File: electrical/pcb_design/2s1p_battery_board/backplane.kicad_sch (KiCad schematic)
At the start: 37 parts, among them J1 TE_Connectivity_7-5530843-7, J10 TE_Connectivity_7-5530843-7, J11 TE_Connectivity_7-5530843-7, J12 TE_Connectivity_7-5530843-7, J13 TE_Connectivity_7-5530843-7, J14 TE_Connectivity_7-5530843-7, J15 TE_Connectivity_7-5530843-7, J16 TE_Connectivity_7-5530843-7, J2 TE_Connectivity_7-5530843-7, J3 TE_Connectivity_7-5530843-7, J4 TE_Connectivity_7-5530843-7, J5 TE_Connectivity_7-5530843-7, J6 TE_Connectivity_7-5530843-7, J7 TE_Connectivity_7-5530843-7, J8 TE_Connectivity_7-5530843-7, J9 TE_Connectivity_7-5530843-7, U3 TCAN330

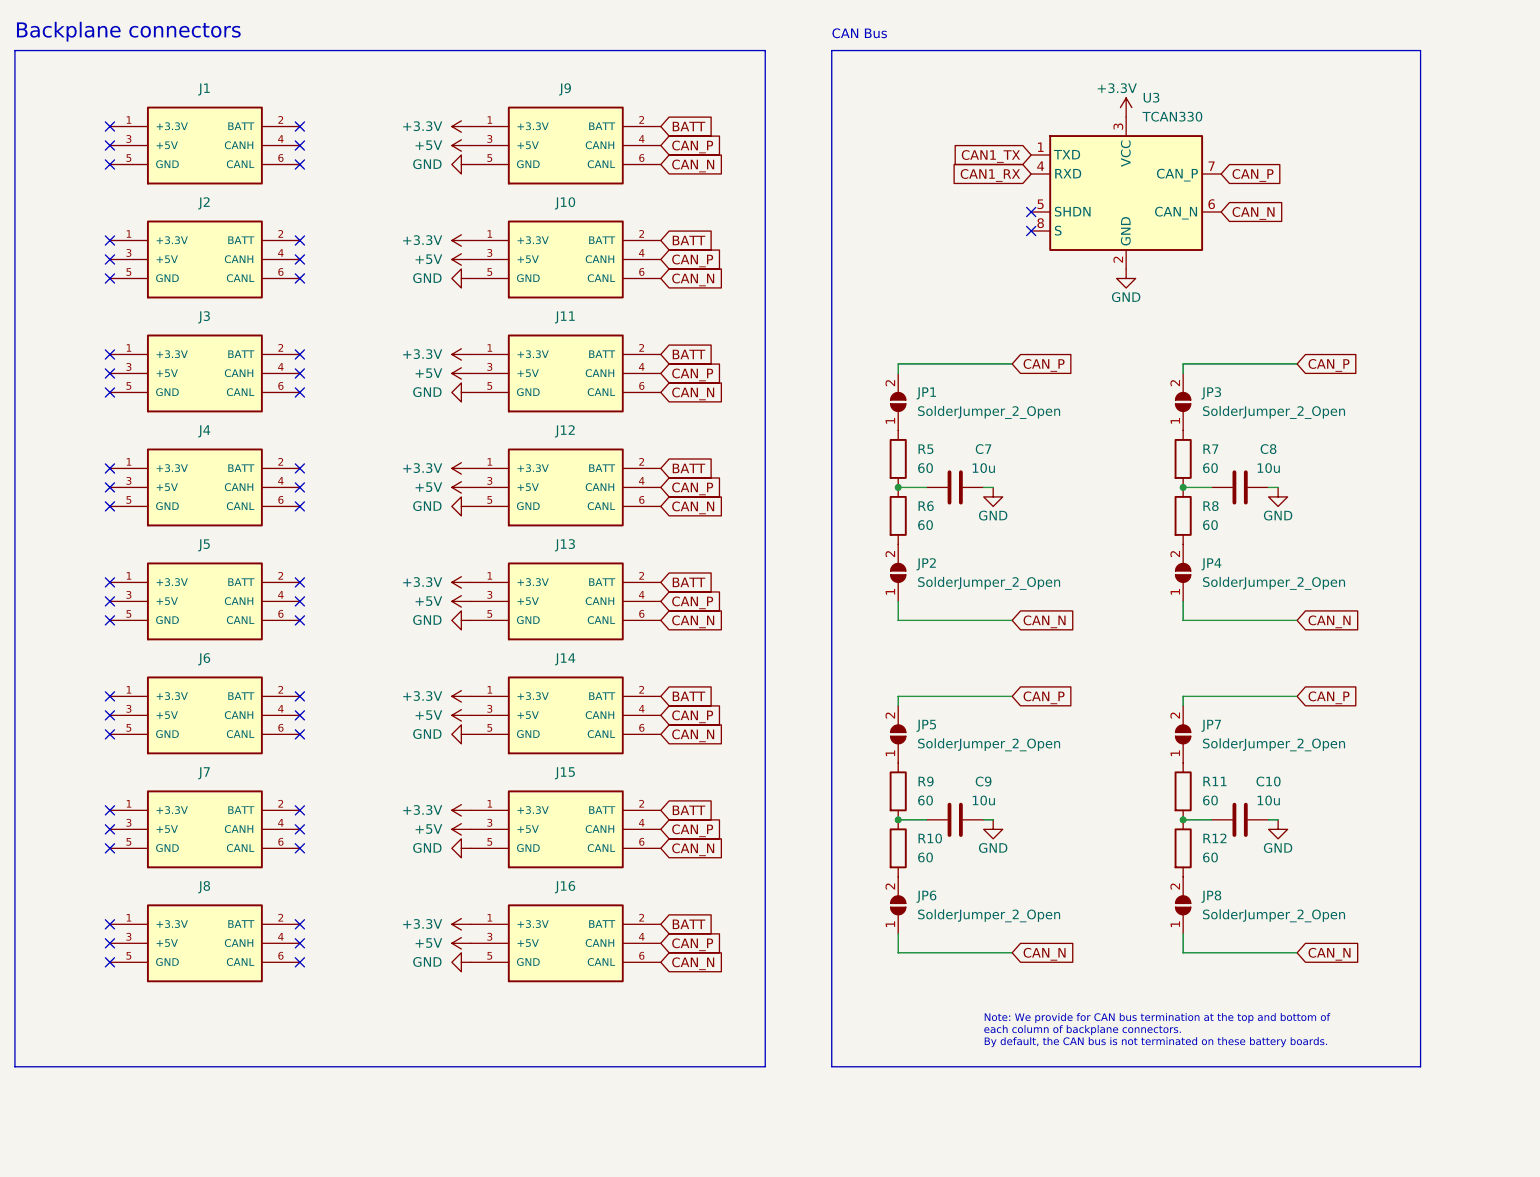
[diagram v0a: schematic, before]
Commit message: Checkpointing work on battery boards
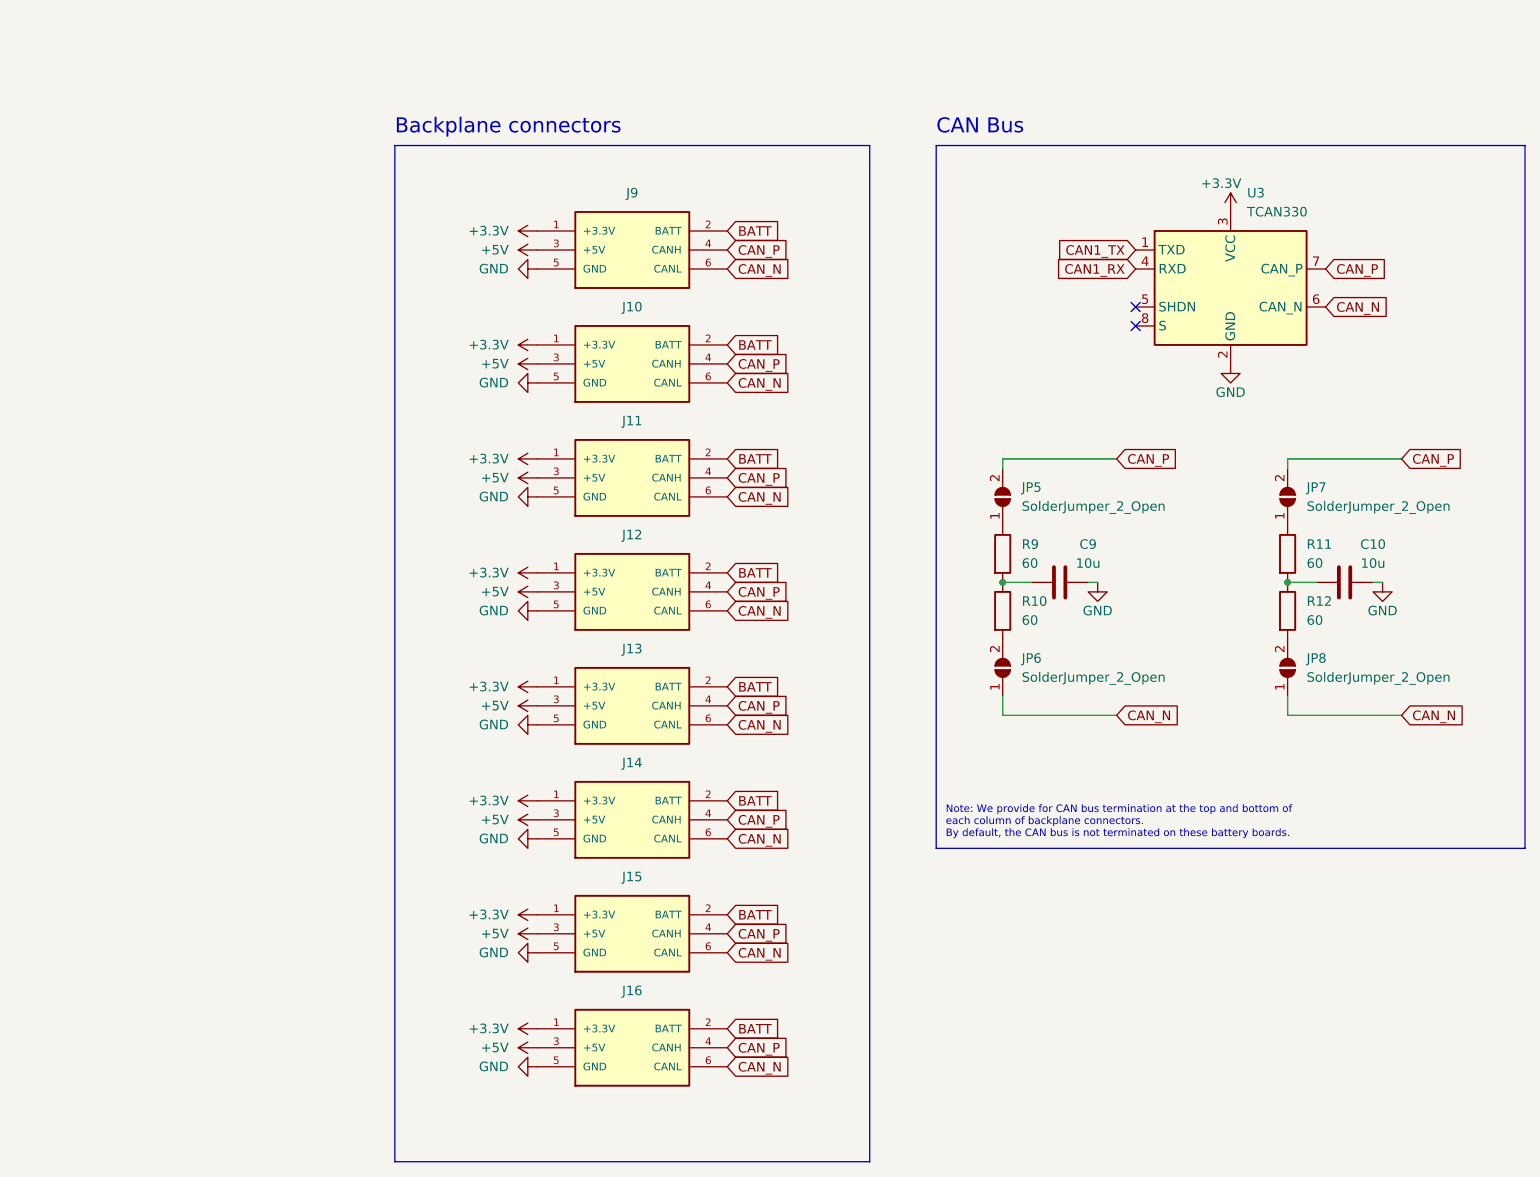
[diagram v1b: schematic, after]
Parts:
- removed C7, C8: 10u, Capacitor_SMD:C_0603_1608Metric, symbol Device:C
- removed J1, J2, J3, J4, J5, J6, J7, J8: TE_Connectivity_7-5530843-7, footprints:TE_Connectivity_7-5530843-7, symbol TVSC:Backplane_Connector_Consumer
- removed JP1, JP2, JP3, JP4: SolderJumper_2_Open, Jumper:SolderJumper-2_P1.3mm_Bridged_RoundedPad1.0x1.5mm, symbol Jumper:SolderJumper_2_Open
- removed R5, R6, R7, R8: 60, Resistor_SMD:R_0402_1005Metric, symbol Device:R
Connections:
- no-connect marks 50 -> 2
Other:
- moved on the sheet: C10, C9, J10, J11, J12, J13, J14, J15, J16, J9, JP5, JP6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
